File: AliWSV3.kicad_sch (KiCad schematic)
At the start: 12 parts, among them CON1 JTAG-2X3-1.27MM-HDR, J1 WSCE, M1 MR256A08BS035, U1 EPM240T100, U2 MX29LV640ETTI-70G

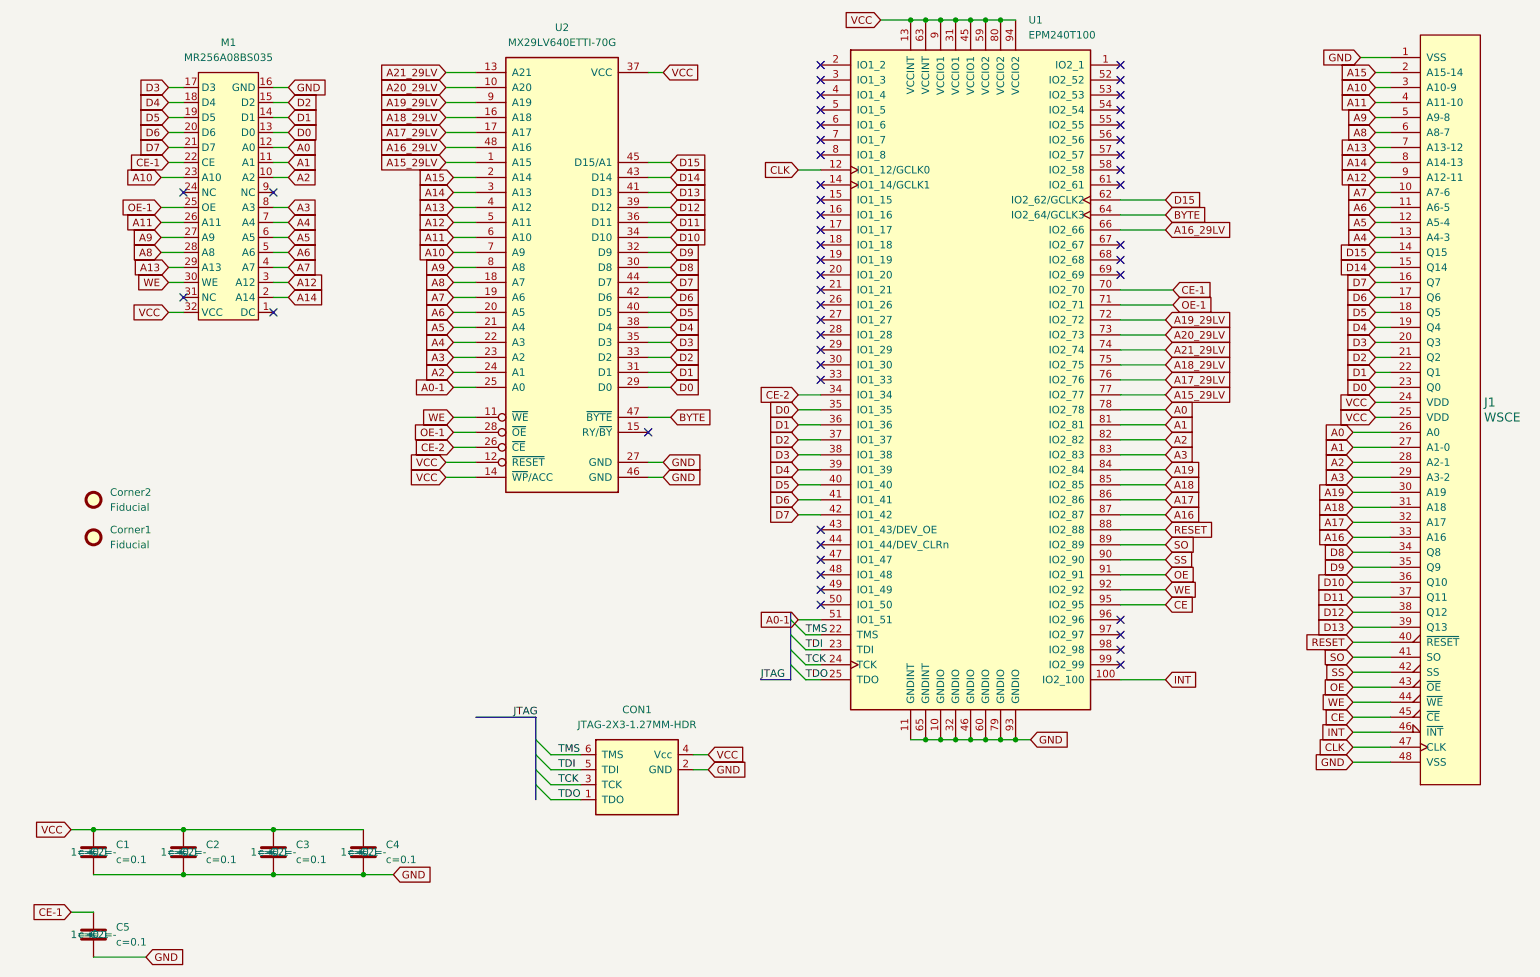
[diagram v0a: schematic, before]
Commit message: Added Gerbers and made some slight changes to PCB
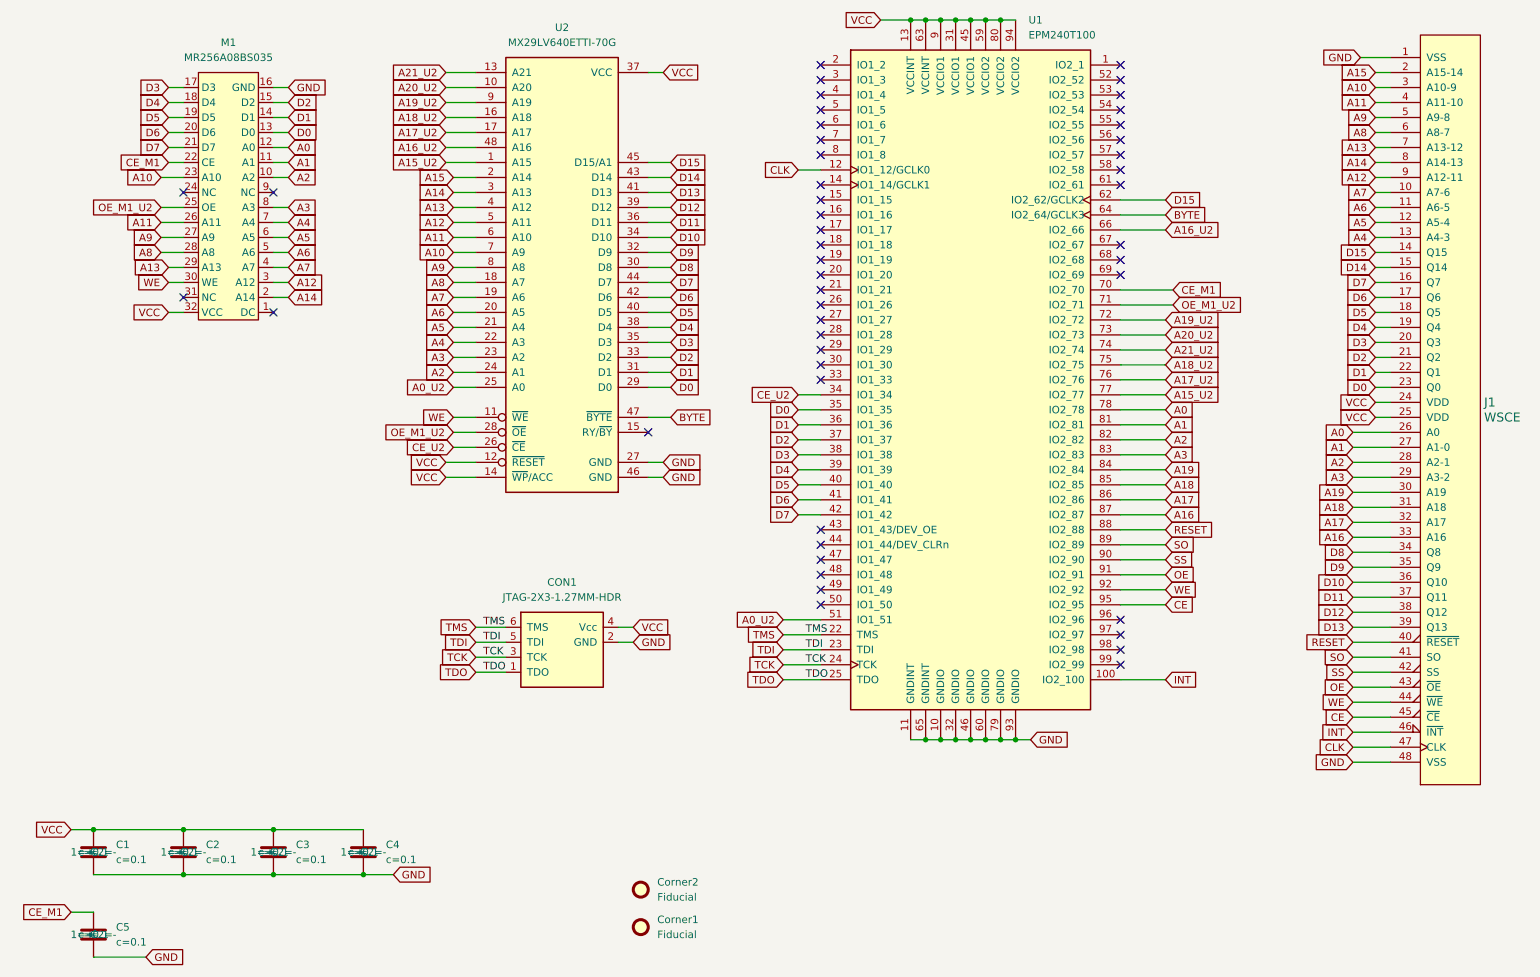
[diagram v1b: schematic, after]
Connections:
- net A0-1 renamed A0_U2
- net A15_29LV renamed A15_U2
- net A16_29LV renamed A16_U2
- net A17_29LV renamed A17_U2
- net A18_29LV renamed A18_U2
- net A19_29LV renamed A19_U2
- net A20_29LV renamed A20_U2
- net A21_29LV renamed A21_U2
- net CE-1 renamed CE_M1
- net CE-2 renamed CE_U2
- net OE-1 renamed OE_M1_U2
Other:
- moved on the sheet: CON1, Corner1, Corner2
